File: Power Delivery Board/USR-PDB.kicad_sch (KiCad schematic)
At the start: 40 parts, among them IC1 LM7805ECT, IC2 LM7805ECT, J1 XT90PW-M, U10 Anderson PP45 Vert. 2x1, U11 Anderson PP45 Vert. 2x1, U12 Anderson PP45 Vert. 2x1, U14 MCP3002-I/P, U17 AMS1117-3.3, U2 Anderson PP45 Vert. 2x1, U3 Anderson PP45 Vert. 2x1, U4 Anderson PP45 Vert. 2x1, U5 Anderson PP45 Vert. 2x1, U6 Anderson PP45 Vert. 2x1, U7 LM2676T-12_NOPB

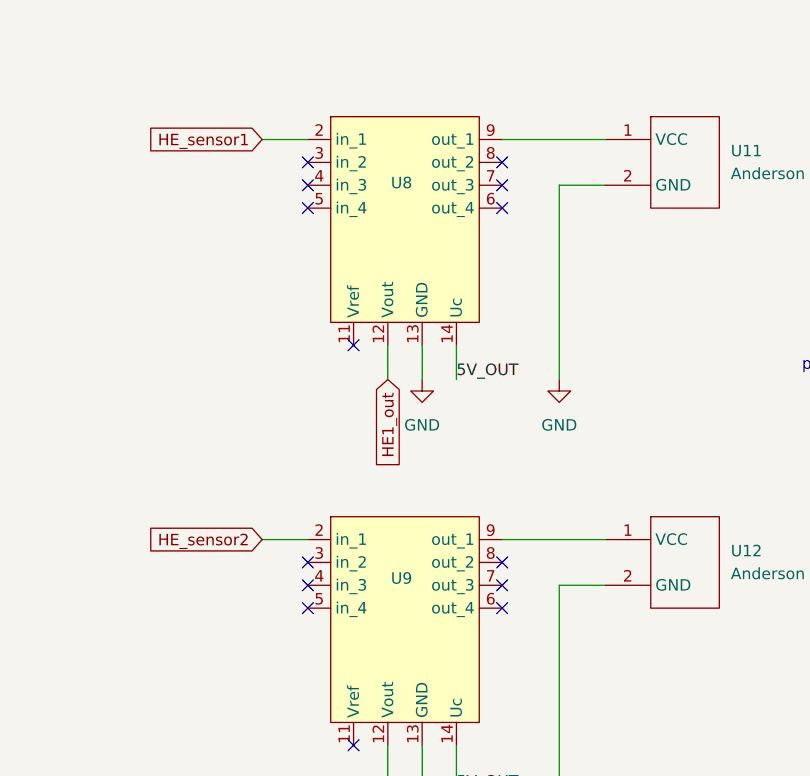
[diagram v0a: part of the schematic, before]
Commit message: Complete redesign of PDB pcb
AAAAAAAAAAAAAAAAAAAAAAAAAAAAAAAAAAAAAAAAAAAA
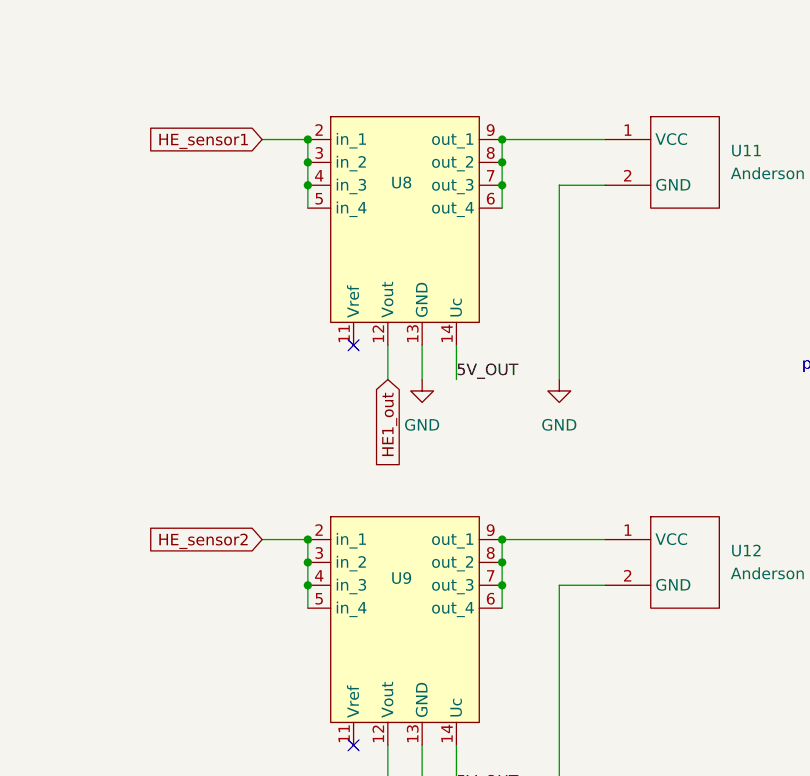
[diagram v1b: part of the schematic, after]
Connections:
- net HE_sensor1: now also U8.3 (in_2), U8.4 (in_3), U8.5 (in_4)
- net HE_sensor2: now also U9.3 (in_2), U9.4 (in_3), U9.5 (in_4)
- net at U12.1 (VCC), U9.9 (out_1): now also U9.6 (out_4), U9.7 (out_3), U9.8 (out_2)
- net at U8.6 (out_4): now also U11.1 (VCC), U8.7 (out_3), U8.8 (out_2), U8.9 (out_1)
- no-connect marks 15 -> 3
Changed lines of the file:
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@@
+	)
+	(junction
+		(at 147.32 81.28)
+		(diameter 0)
+		(color 0 0 0 0)
 	)
 	(junction
@@
 	)
 	(junction
+		(at 168.91 83.82)
+		(diameter 0)
+		(color 0 0 0 0)
+	)
+	(junction
+		(at 168.91 78.74)
+		(diameter 0)
+		(color 0 0 0 0)
+	)
+	(junction
+		(at 168.91 34.29)
+		(diameter 0)
+		(color 0 0 0 0)
+	)
+	(junction
 		(at 29.21 106.68)
 		(diameter 0)
@@
 	)
 	(junction
+		(at 147.32 36.83)
+		(diameter 0)
+		(color 0 0 0 0)
+	)
+	(junction
 		(at 285.75 132.08)
 		(diameter 0)
@@
 	)
 	(junction
+		(at 147.32 83.82)
+		(diameter 0)
+		(color 0 0 0 0)
+	)
+	(junction
 		(at 289.56 219.71)
 		(diameter 0)
@@
 	)
 	(junction
+		(at 168.91 36.83)
+		(diameter 0)
+		(color 0 0 0 0)
+	)
+	(junction
 		(at 303.53 104.14)
 		(diameter 0)
@@
 	)
 	(junction
+		(at 147.32 78.74)
+		(diameter 0)
+		(color 0 0 0 0)
+	)
+	(junction
 		(at 29.21 143.51)
 		(diameter 0)
@@
 	)
 	(junction
+		(at 147.32 39.37)
+		(diameter 0)
+		(color 0 0 0 0)
+	)
+	(junction
 		(at 31.75 175.26)
 		(diameter 0)
@@
 	)
 	(junction
+		(at 147.32 34.29)
+		(diameter 0)
+		(color 0 0 0 0)
+	)
+	(junction
 		(at 292.1 156.21)
 		(diameter 0)
@@
 	(junction
 		(at 341.63 210.82)
+		(diameter 0)
+		(color 0 0 0 0)
+	)
+	(junction
+		(at 168.91 81.28)
+		(diameter 0)
+		(color 0 0 0 0)
+	)
+	(junction
+		(at 168.91 39.37)
 		(diameter 0)
 		(color 0 0 0 0)
@@
 	)
 	(no_connect
-		(at 147.32 86.36)
-	)
-	(no_connect
-		(at 168.91 86.36)
-	)
-	(no_connect
 		(at 152.4 101.6)
 	)
-	(no_connect
-		(at 147.32 83.82)
-	)
-	(no_connect
-		(at 147.32 36.83)
-	)
-	(no_connect
-		(at 168.91 83.82)
-	)
-	(no_connect
-		(at 147.32 41.91)
-	)
-	(no_connect
-		(at 168.91 39.37)
-	)
-	(no_connect
-		(at 147.32 39.37)
-	)
-	(no_connect
-		(at 147.32 81.28)
-	)
-	(no_connect
-		(at 168.91 81.28)
-	)
-	(no_connect
-		(at 168.91 41.91)
-	)
-	(no_connect
-		(at 168.91 36.83)
+	(wire
+		(pts
+			(xy 168.91 39.37) (xy 168.91 41.91)
+		)
+		(stroke
+			(width 0)
+			(type default)
+		)
 	)
 	(wire
@@
 	(wire
 		(pts
+			(xy 147.32 81.28) (xy 147.32 83.82)
+		)
+		(stroke
+			(width 0)
+			(type default)
+		)
+	)
+	(wire
+		(pts
 			(xy 312.42 156.21) (xy 312.42 173.99)
 		)
@@
 	(wire
 		(pts
+			(xy 168.91 78.74) (xy 168.91 81.28)
+		)
+		(stroke
+			(width 0)
+			(type default)
+		)
+	)
+	(wire
+		(pts
 			(xy 31.75 120.65) (xy 41.91 120.65)
 		)
@@
 	(wire
 		(pts
+			(xy 168.91 83.82) (xy 168.91 86.36)
+		)
+		(stroke
+			(width 0)
+			(type default)
+		)
+	)
+	(wire
+		(pts
 			(xy 180.34 83.82) (xy 175.26 83.82)
 		)
@@
 	(wire
 		(pts
+			(xy 168.91 81.28) (xy 168.91 83.82)
+		)
+		(stroke
+			(width 0)
+			(type default)
+		)
+	)
+	(wire
+		(pts
 			(xy 340.36 213.36) (xy 345.44 213.36)
 		)
@@
 	(wire
 		(pts
+			(xy 168.91 34.29) (xy 168.91 36.83)
+		)
+		(stroke
+			(width 0)
+			(type default)
+		)
+	)
+	(wire
+		(pts
 			(xy 29.21 106.68) (xy 29.21 125.73)
 		)
@@
 	(wire
 		(pts
+			(xy 147.32 78.74) (xy 147.32 81.28)
+		)
+		(stroke
+			(width 0)
+			(type default)
+		)
+	)
+	(wire
+		(pts
 			(xy 31.75 157.48) (xy 41.91 157.48)
 		)
@@
 	(wire
 		(pts
+			(xy 147.32 39.37) (xy 147.32 41.91)
+		)
+		(stroke
+			(width 0)
+			(type default)
+		)
+	)
+	(wire
+		(pts
 			(xy 29.21 143.51) (xy 29.21 162.56)
 		)
@@
 	(wire
 		(pts
+			(xy 147.32 83.82) (xy 147.32 86.36)
+		)
+		(stroke
+			(width 0)
+			(type default)
+		)
+	)
+	(wire
+		(pts
 			(xy 345.44 213.36) (xy 349.25 213.36)
 		)
@@
 	(wire
 		(pts
+			(xy 147.32 34.29) (xy 147.32 36.83)
+		)
+		(stroke
+			(width 0)
+			(type default)
+		)
+	)
+	(wire
+		(pts
 			(xy 196.85 229.87) (xy 199.39 229.87)
 		)
@@
 	(wire
 		(pts
+			(xy 168.91 36.83) (xy 168.91 39.37)
+		)
+		(stroke
+			(width 0)
+			(type default)
+		)
+	)
+	(wire
+		(pts
 			(xy 312.42 104.14) (xy 312.42 121.92)
 		)
@@
 		)
 		(stroke
+			(width 0)
+			(type default)
+		)
+	)
+	(wire
+		(pts
+			(xy 147.32 36.83) (xy 147.32 39.37)
+		)
+		(stroke
